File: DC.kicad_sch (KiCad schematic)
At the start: 89 parts, among them J1 348302001, J2 348302001, J3 757570141, J4 PPTC021LFBN-RC, U6 MCP2551-I-P, U7 NUCLEO-F302R8, U8 100DP6T1B1M1QEH

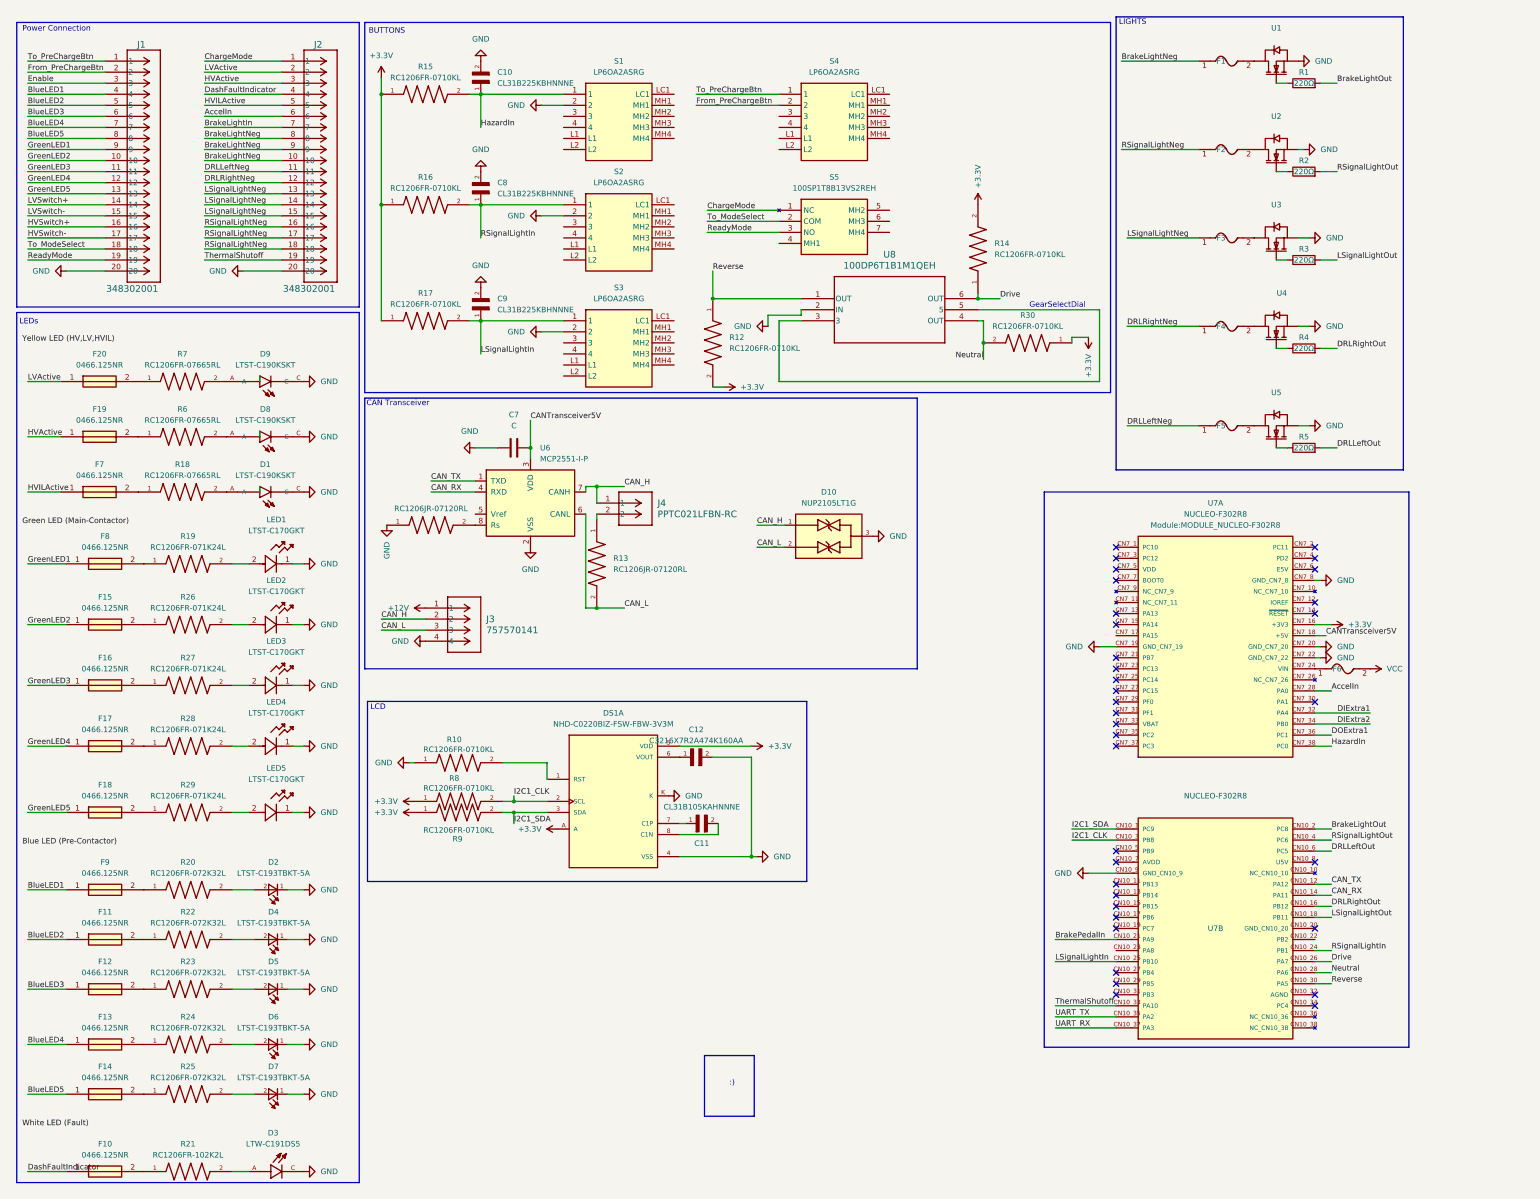
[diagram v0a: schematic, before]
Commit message: VCU revisions, last review still to be done
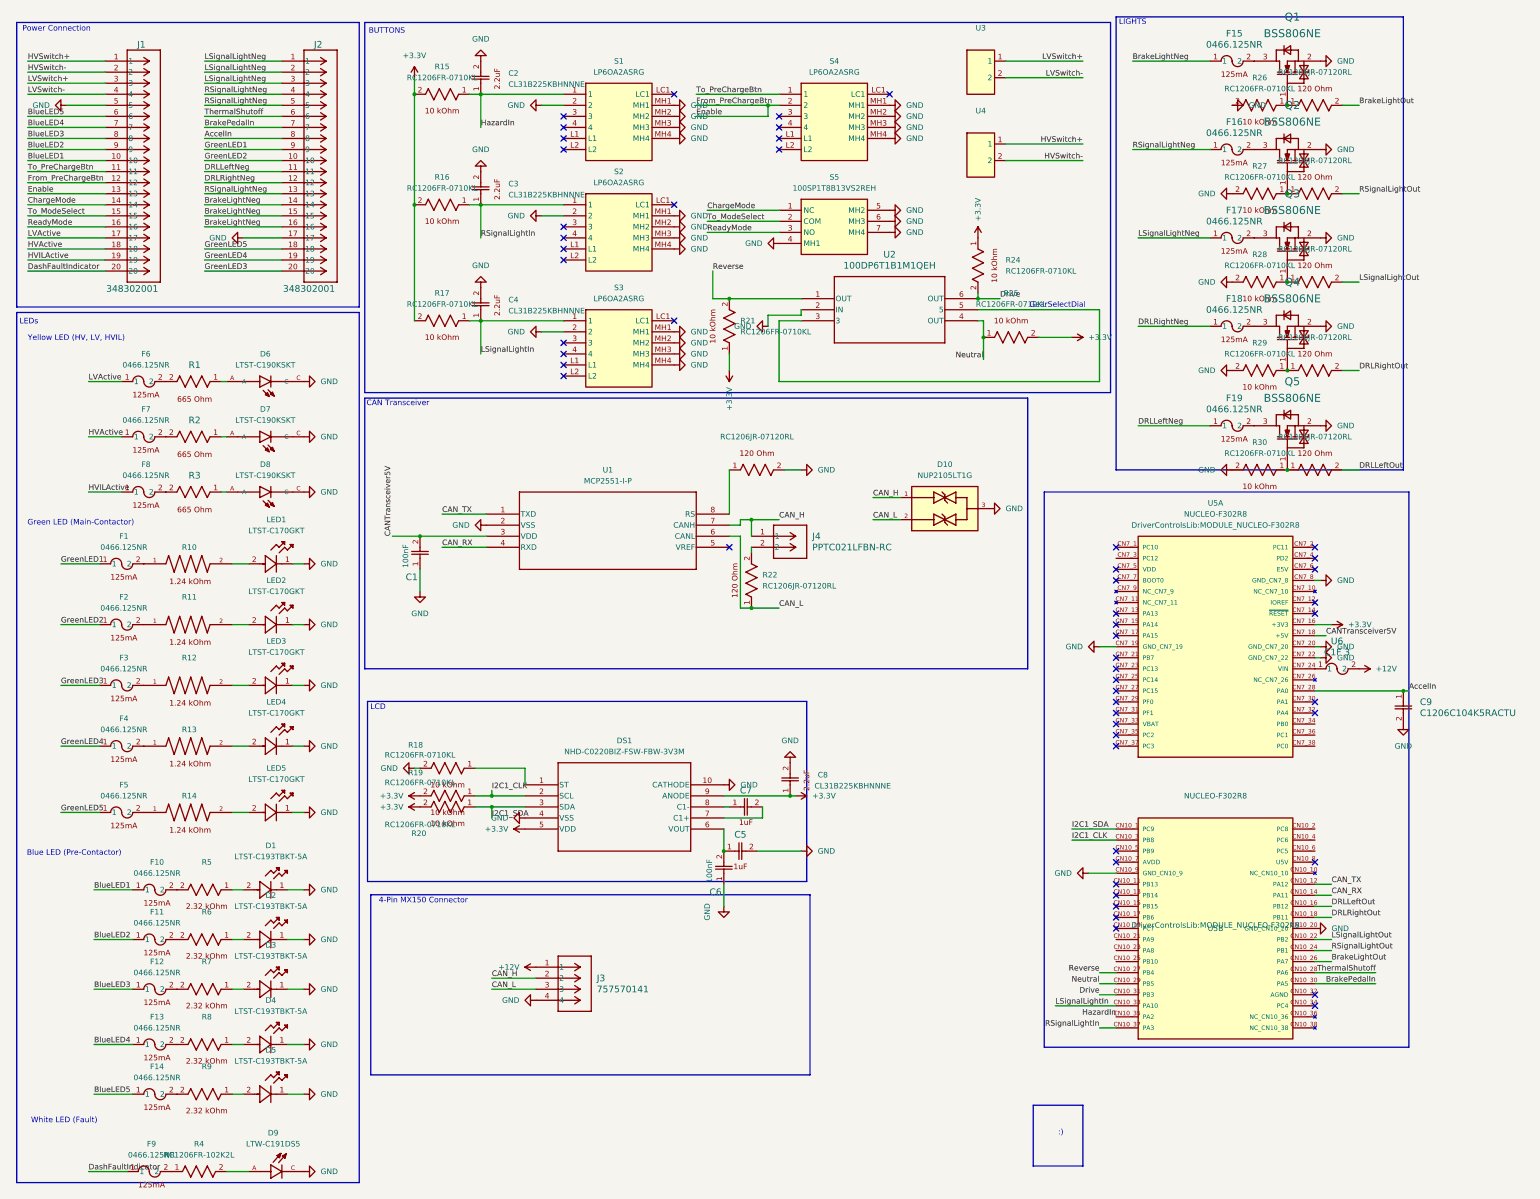
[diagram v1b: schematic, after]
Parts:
- removed C11: CL31B105KAHNNNE, Capacitor_SMD:CAPC3216X180N, symbol CL31B105KAHNNNE:CL31B105KAHNNNE
- removed C12: C3216X7R2A474K160AA, Capacitor_SMD:CAPC3216X180N, symbol C3216X7R2A474K160AA:C3216X7R2A474K160AA
- removed C7: C, DriverControlsLib:CAP-TH_L6.0-W3.5-P7.50-D1.0, symbol DC_Parts:C
- removed F1, F2, F3, F6: ~, DriverControlsLib:FUSE-TH_BD5.4-W22.5-P27.5-D0.8, symbol DC_Parts:0001.2511.TR
- removed F4, F5: ~, Fuse:FUSC3215X66N, symbol DC_Parts:0001.2511.TR
- removed J4: PPTC021LFBN-RC, Connector:CONN2_LFBN-RC_SUL, symbol 2026-02-13_01-22-03:PPTC021LFBN-RC
- removed R1, R2, R3, R4, R5: 220Ω, Resistor_SMD:RESC3216X70N, symbol DC_Parts:R
- removed R18, R6, R7: RC1206FR-07665RL, Resistor_SMD:RESC3116X65N, symbol RC1206FR-07665RL:RC1206FR-07665RL
- removed S1, S2, S3, S4: LP6OA2ASRG, Button_Switch_SMD:LP6OA2ASRG, symbol LP6OA2ASRG:LP6OA2ASRG
- removed S5: 100SP1T8B13VS2REH, Button_Switch_SMD:100SP1T8B13VS2REH, symbol 100SP1T8B13VS2REH:100SP1T8B13VS2REH
- removed U1, U2, U3, U4, U5: ~, Battery:TO254P470X1016X2019-3P, symbol DC_Parts:FQP30N06L
- removed U8: 100DP6T1B1M1QEH, MiscellaneousLibrary:TO_1M1QEH_EWI, symbol Gear-Select-Dial:100DP6T1B1M1QEH
- added C1, C6, C9: C1206C104K5RACTU, DriverControlsLib:CAPC340180_88N_KEM, symbol DriverControlsLib:C1206C104K5RACTU
- added C5, C7: CL31B105KAHNNNE, DriverControlsLib:CAP_CL31_SAM, symbol DriverControlsLib:CL31B105KAHNNNE
- added C8: CL31B225KBHNNNE, DriverControlsLib:CAP_CL31_SAM, symbol DriverControlsLib:CL31B225KBHNNNE
- added F15, F16, F17, F18, F19: 0466.125NR, DriverControlsLib:0466Series_LTF, symbol DriverControlsLib:0466.125NR
- added J4: PPTC021LFBN-RC, DriverControlsLib:CONN2_LFBN-RC_SUL, symbol DriverControlsLib:PPTC021LFBN-RC
- added Q1, Q2, Q3, Q4, Q5: BSS806NE, DriverControlsLib:SOT95P240X110-3N-1-V1, symbol DriverControlsLib:BSS806NE
- added R1, R2, R3: RC1206FR-07665RL, DriverControlsLib:RC1206N_YAG, symbol DriverControlsLib:RC1206FR-07665RL
- added R26, R27, R28, R29, R30: RC1206FR-0710KL, DriverControlsLib:RC1206N_YAG, symbol DriverControlsLib:RC1206FR-0710KL
- added R31, R32, R33, R34, R35: RC1206JR-07120RL, DriverControlsLib:RC1206N_YAG, symbol DriverControlsLib:RC1206JR-07120RL
- added S1, S2, S3, S4: LP6OA2ASRG, DriverControlsLib:LP6OA2ASRG, symbol DriverControlsLib:LP6OA2ASRG
- added S5: 100SP1T8B13VS2REH, DriverControlsLib:100SP1T8B13VS2REH, symbol DriverControlsLib:100SP1T8B13VS2REH
- added U2: 100DP6T1B1M1QEH, DriverControlsLib:TO_1M1QEH_EWI, symbol DriverControlsLib:100DP6T1B1M1QEH
- added U3: ~, DriverControlsLib:LV_Switch, symbol DriverControlsLib:LV_Switch
- added U4: ~, DriverControlsLib:HV_Switch, symbol DriverControlsLib:HV_Switch
- added U6: C1F 3, DriverControlsLib:C1_BEL, symbol DriverControlsLib:C1F_3
- C2: renamed from C10; footprint Capacitor_SMD:CAPC3216X180N -> DriverControlsLib:CAP_CL31_SAM; symbol CL31B225KBHNNNE:CL31B225KBHNNNE -> DriverControlsLib:CL31B225KBHNNNE
- C3: renamed from C8; footprint Capacitor_SMD:CAPC3216X180N -> DriverControlsLib:CAP_CL31_SAM; symbol CL31B225KBHNNNE:CL31B225KBHNNNE -> DriverControlsLib:CL31B225KBHNNNE
- C4: renamed from C9; footprint Capacitor_SMD:CAPC3216X180N -> DriverControlsLib:CAP_CL31_SAM; symbol CL31B225KBHNNNE:CL31B225KBHNNNE -> DriverControlsLib:CL31B225KBHNNNE
- D1: renamed from D2; footprint Fuse:Fuse_0603_1608Metric -> DriverControlsLib:LED_LTST-C_LTO; symbol LTST-C193TBKT-5A:LTST-C193TBKT-5A -> DriverControlsLib:LTST-C193TBKT-5A
- D2: renamed from D4; footprint Fuse:Fuse_0603_1608Metric -> DriverControlsLib:LED_LTST-C_LTO; symbol LTST-C193TBKT-5A:LTST-C193TBKT-5A -> DriverControlsLib:LTST-C193TBKT-5A
- D3: renamed from D5; footprint Fuse:Fuse_0603_1608Metric -> DriverControlsLib:LED_LTST-C_LTO; symbol LTST-C193TBKT-5A:LTST-C193TBKT-5A -> DriverControlsLib:LTST-C193TBKT-5A
- D4: renamed from D6; footprint Fuse:Fuse_0603_1608Metric -> DriverControlsLib:LED_LTST-C_LTO; symbol LTST-C193TBKT-5A:LTST-C193TBKT-5A -> DriverControlsLib:LTST-C193TBKT-5A
- D5: renamed from D7; footprint Fuse:Fuse_0603_1608Metric -> DriverControlsLib:LED_LTST-C_LTO; symbol LTST-C193TBKT-5A:LTST-C193TBKT-5A -> DriverControlsLib:LTST-C193TBKT-5A
- D6: renamed from D9; footprint LED_SMD:LEDM1608X80 -> DriverControlsLib:LEDM1608X80; symbol LTST-C190KSKT:LTST-C190KSKT -> DriverControlsLib:LTST-C190KSKT
- D7: renamed from D8; footprint LED_SMD:LEDM1608X80 -> DriverControlsLib:LEDM1608X80; symbol LTST-C190KSKT:LTST-C190KSKT -> DriverControlsLib:LTST-C190KSKT
- D8: renamed from D1; footprint LED_SMD:LEDM1608X80 -> DriverControlsLib:LEDM1608X80; symbol LTST-C190KSKT:LTST-C190KSKT -> DriverControlsLib:LTST-C190KSKT
- D9: renamed from D3; footprint LED_SMD:LEDC1608X65N -> DriverControlsLib:LEDC1608X65N; symbol LTW-C191DS5:LTW-C191DS5 -> DriverControlsLib:LTW-C191DS5
- DS1: footprint Display:LCD_NHD-C0220BIZ-FSW-FBW-3V3M -> DriverControlsLib:NHD-C0220BIZ-FSW-FBW-3V3M_NDI; symbol NHD-C0220BIZ-FSW-FBW-3V3M:NHD-C0220BIZ-FSW-FBW-3V3M -> DriverControlsLib:NHD-C0220BIZ-FSW-FBW-3V3M
- F1: renamed from F8; footprint Fuse:FUSC3215X66N -> DriverControlsLib:0466Series_LTF; symbol 0466_125NR:0466.125NR -> DriverControlsLib:0466.125NR
- F10: renamed from F9; footprint Fuse:FUSC3215X66N -> DriverControlsLib:0466Series_LTF; symbol 0466_125NR:0466.125NR -> DriverControlsLib:0466.125NR
- F11, F12, F13, F14: footprint Fuse:FUSC3215X66N -> DriverControlsLib:0466Series_LTF; symbol 0466_125NR:0466.125NR -> DriverControlsLib:0466.125NR
- F2: renamed from F15; footprint Fuse:FUSC3215X66N -> DriverControlsLib:0466Series_LTF; symbol 0466_125NR:0466.125NR -> DriverControlsLib:0466.125NR
- F3: renamed from F16; footprint Fuse:FUSC3215X66N -> DriverControlsLib:0466Series_LTF; symbol 0466_125NR:0466.125NR -> DriverControlsLib:0466.125NR
- F4: renamed from F17; footprint Fuse:FUSC3215X66N -> DriverControlsLib:0466Series_LTF; symbol 0466_125NR:0466.125NR -> DriverControlsLib:0466.125NR
- F5: renamed from F18; footprint Fuse:FUSC3215X66N -> DriverControlsLib:0466Series_LTF; symbol 0466_125NR:0466.125NR -> DriverControlsLib:0466.125NR
- F6: renamed from F20; footprint Fuse:FUSC3215X66N -> DriverControlsLib:0466Series_LTF; symbol 0466_125NR:0466.125NR -> DriverControlsLib:0466.125NR
- F7: renamed from F19; footprint Fuse:FUSC3215X66N -> DriverControlsLib:0466Series_LTF; symbol 0466_125NR:0466.125NR -> DriverControlsLib:0466.125NR
- F8: renamed from F7; footprint Fuse:FUSC3215X66N -> DriverControlsLib:0466Series_LTF; symbol 0466_125NR:0466.125NR -> DriverControlsLib:0466.125NR
- F9: renamed from F10; footprint Fuse:FUSC3215X66N -> DriverControlsLib:0466Series_LTF; symbol 0466_125NR:0466.125NR -> DriverControlsLib:0466.125NR
- J1, J2: footprint Connector_Molex:CONN_SD-34829-001_20_ST_MOL -> DriverControlsLib:CONN_SD-34829-001_20_ST_MOL; symbol MX150_sym:348302001 -> DriverControlsLib:348302001
- J3: footprint Connector_Molex:CONN_SD-75757-010_1X4_F11p20_MOL -> DriverControlsLib:CONN_SD-75757-010_1X4_F11p20_MOL; symbol 2026-02-11_03-05-32:757570141 -> DriverControlsLib:757570141
- LED1, LED2, LED3, LED4, LED5: footprint LED_SMD:LED_LTST-C170GKT_LTO -> DriverControlsLib:LED_LTST-C170GKT_LTO; symbol 2026-02-10_18-36-51:LTST-C170GKT -> DriverControlsLib:LTST-C170GKT
- R10: renamed from R19; footprint Resistor_SMD:RESC3116X65N -> DriverControlsLib:RESC3116X65N; symbol RC1206FR-071K24L:RC1206FR-071K24L -> DriverControlsLib:RC1206FR-071K24L
- R11: renamed from R26; footprint Resistor_SMD:RESC3116X65N -> DriverControlsLib:RESC3116X65N; symbol RC1206FR-071K24L:RC1206FR-071K24L -> DriverControlsLib:RC1206FR-071K24L
- R12: renamed from R27; footprint Resistor_SMD:RESC3116X65N -> DriverControlsLib:RESC3116X65N; symbol RC1206FR-071K24L:RC1206FR-071K24L -> DriverControlsLib:RC1206FR-071K24L
- R13: renamed from R28; footprint Resistor_SMD:RESC3116X65N -> DriverControlsLib:RESC3116X65N; symbol RC1206FR-071K24L:RC1206FR-071K24L -> DriverControlsLib:RC1206FR-071K24L
- R14: renamed from R29; footprint Resistor_SMD:RESC3116X65N -> DriverControlsLib:RESC3116X65N; symbol RC1206FR-071K24L:RC1206FR-071K24L -> DriverControlsLib:RC1206FR-071K24L
- R15, R16, R17: footprint Resistor_SMD:RESC3116X65N -> DriverControlsLib:RC1206N_YAG; symbol RC1206FR-0710KL:RC1206FR-0710KL -> DriverControlsLib:RC1206FR-0710KL
- R18: renamed from R10; footprint Resistor_SMD:RESC3116X65N -> DriverControlsLib:RC1206N_YAG; symbol RC1206FR-0710KL:RC1206FR-0710KL -> DriverControlsLib:RC1206FR-0710KL
- R19: renamed from R8; footprint Resistor_SMD:RESC3116X65N -> DriverControlsLib:RC1206N_YAG; symbol RC1206FR-0710KL:RC1206FR-0710KL -> DriverControlsLib:RC1206FR-0710KL
- R20: renamed from R9; footprint Resistor_SMD:RESC3116X65N -> DriverControlsLib:RC1206N_YAG; symbol RC1206FR-0710KL:RC1206FR-0710KL -> DriverControlsLib:RC1206FR-0710KL
- R21: renamed from R12; footprint MiscellaneousLibrary:RESC3116X65N -> DriverControlsLib:RC1206N_YAG; symbol RC1206FR-0710KL:RC1206FR-0710KL -> DriverControlsLib:RC1206FR-0710KL
- R22: renamed from R13; footprint Resistor_SMD:RESC3116X65N -> DriverControlsLib:RC1206N_YAG; symbol RC1206JR-07120RL:RC1206JR-07120RL -> DriverControlsLib:RC1206JR-07120RL
- R23: renamed from R11; footprint Resistor_SMD:RESC3116X65N -> DriverControlsLib:RC1206N_YAG; symbol RC1206JR-07120RL:RC1206JR-07120RL -> DriverControlsLib:RC1206JR-07120RL
- R24: renamed from R14; footprint MiscellaneousLibrary:RESC3116X65N -> DriverControlsLib:RC1206N_YAG; symbol RC1206FR-0710KL:RC1206FR-0710KL -> DriverControlsLib:RC1206FR-0710KL
- R25: renamed from R30; footprint MiscellaneousLibrary:RESC3116X65N -> DriverControlsLib:RC1206N_YAG; symbol RC1206FR-0710KL:RC1206FR-0710KL -> DriverControlsLib:RC1206FR-0710KL
- R4: renamed from R21; footprint Resistor_SMD:RESC3116X65N -> DriverControlsLib:RES_RC1206_YAG; symbol RC1206FR-102K2L:RC1206FR-102K2L -> DriverControlsLib:RC1206FR-102K2L
- R5: renamed from R20; footprint Resistor_SMD:RESC3116X65N -> DriverControlsLib:RC1206N_YAG; symbol RC1206FR-072K32L:RC1206FR-072K32L -> DriverControlsLib:RC1206FR-072K32L
- R6: renamed from R22; footprint Resistor_SMD:RESC3116X65N -> DriverControlsLib:RC1206N_YAG; symbol RC1206FR-072K32L:RC1206FR-072K32L -> DriverControlsLib:RC1206FR-072K32L
- R7: renamed from R23; footprint Resistor_SMD:RESC3116X65N -> DriverControlsLib:RC1206N_YAG; symbol RC1206FR-072K32L:RC1206FR-072K32L -> DriverControlsLib:RC1206FR-072K32L
- R8: renamed from R24; footprint Resistor_SMD:RESC3116X65N -> DriverControlsLib:RC1206N_YAG; symbol RC1206FR-072K32L:RC1206FR-072K32L -> DriverControlsLib:RC1206FR-072K32L
- R9: renamed from R25; footprint Resistor_SMD:RESC3116X65N -> DriverControlsLib:RC1206N_YAG; symbol RC1206FR-072K32L:RC1206FR-072K32L -> DriverControlsLib:RC1206FR-072K32L
- U1: renamed from U6; footprint Package_DIP:DIP-8_W7.62mm -> DriverControlsLib:PDIP8_300MC_MCH; symbol DC_Parts:MCP2551-I-P -> DriverControlsLib:MCP2551-I_P
- U5: renamed from U7; footprint Module:MODULE_NUCLEO-F302R8 -> DriverControlsLib:MODULE_NUCLEO-F302R8; symbol DC_Parts:NUCLEO-F302R8 -> DriverControlsLib:NUCLEO-F302R8
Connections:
- net BrakeLightIn is gone; now on net BrakePedalIn: J2.7
- net From_PreChargeBtn is gone; now on net HVSwitch-: J1.2
- net UART_RX is gone; now on net RSignalLightIn: U5.CN10_37 (PA3)
- net UART_TX is gone; now on net HazardIn: U5.CN10_35 (PA2)
- net +12V: now also U6.2
- net +3.3V: now also DS1.9 (ANODE), R15.2, R16.2, R17.2, R19.2, R20.2, R21.1, R24.1, R25.2, C8.1; no longer DS1.A, R15.1, R16.1, R17.1, R19.1, R20.1, R21.2, R24.2, R25.1
- net AccelIn: now also J2.8, C9.1; no longer J2.6
- net BlueLED1: now also J1.10; no longer J1.4
- net BlueLED2: now also J1.9; no longer J1.5
- net BlueLED3: now also J1.8; no longer J1.6
- net BlueLED5: now also J1.6; no longer J1.8
- net BrakeLightNeg: now also J2.14, J2.15, J2.16, F15.1; no longer J2.10, J2.8, J2.9
- net BrakeLightOut: now also U5.CN10_26 (PA7), R31.2; no longer U5.CN10_2 (PC8)
- net BrakePedalIn: now also U5.CN10_30 (PA5); no longer U5.CN10_21 (PA9)
- net CANTransceiver5V: now also C1.2
- net CAN_H: now also J4.1
- net CAN_L: now also R22.1; no longer R22.2
- net ChargeMode: now also J1.14, S5.1 (NC); no longer J2.1
- net DRLLeftNeg: now also F19.1
- net DRLLeftOut: now also U5.CN10_16 (PB12), R35.2; no longer U5.CN10_6 (PC5)
- net DRLRightNeg: now also F18.1
- net DRLRightOut: now also U5.CN10_18 (PB11), R34.2; no longer U5.CN10_16 (PB12)
- net DashFaultIndicator: now also J1.20; no longer J2.4
- net Drive: now also R24.2, U5.CN10_31 (PB3), U2.6 (OUT); no longer R24.1, U5.CN10_26 (PA7)
- net Enable: now also J1.12, J1.13, S4.2; no longer J1.3
- net GND: now also DS1.10 (CATHODE), J1.5, J2.17, R18.2, R23.2, U5.CN10_20 (GND_CN10_20), C1.1, C5.2, C6.1, C8.2, C9.2, Q1.2 (SOURCE), Q2.2 (SOURCE), Q3.2 (SOURCE), Q4.2 (SOURCE), Q5.2 (SOURCE), R26.2, R27.2, R28.2, R29.2, R30.2, S1.2, S1.MH1, S1.MH2, S1.MH3, S1.MH4, S2.2, S2.MH1, S2.MH2, S2.MH3, S2.MH4, S3.2, S3.MH1, S3.MH2, S3.MH3, S3.MH4, S4.MH1, S4.MH2, S4.MH3, S4.MH4, S5.4 (MH1), S5.5 (MH2), S5.6 (MH3), S5.7 (MH4), U2.2 (IN); no longer DS1.K, J1.20, J2.20, R18.1, R23.1
- net GreenLED1: now also J2.9; no longer J1.9
- net GreenLED2: now also J2.10; no longer J1.10
- net GreenLED3: now also J2.20; no longer J1.11
- net GreenLED4: now also J2.19; no longer J1.12
- net GreenLED5: now also J2.18; no longer J1.13
- net HVActive: now also J1.18; no longer J2.3
- net HVILActive: now also J1.19; no longer J2.5
- net HVSwitch+: now also J1.1, U4.1; no longer J1.16
- net HVSwitch-: now also U4.2; no longer J1.17
- net HazardIn: now also R15.1, S1.1; no longer R15.2, U5.CN7_38 (PC0)
- net I2C1_CLK: now also R19.1; no longer R19.2
- net I2C1_SDA: now also R20.1; no longer R20.2
- net LSignalLightIn: now also R17.1, U5.CN10_33 (PA10), S3.1; no longer R17.2, U5.CN10_25 (PB10)
- net LSignalLightNeg: now also J2.1, J2.2, J2.3, F17.1; no longer J2.13, J2.14, J2.15
- net LSignalLightOut: now also U5.CN10_22 (PB2), R33.2; no longer U5.CN10_18 (PB11)
- net LVActive: now also J1.17; no longer J2.2
- net LVSwitch+: now also J1.3, U3.1; no longer J1.14
- net LVSwitch-: now also J1.4, U3.2; no longer J1.15
- net Neutral: now also R25.1, U5.CN10_29 (PB5), U2.4 (OUT); no longer R25.2, U5.CN10_28 (PA6)
- net RSignalLightIn: now also R16.1, S2.1; no longer R16.2, U5.CN10_24 (PB1)
- net RSignalLightNeg: now also J2.13, J2.4, J2.5, F16.1; no longer J2.16, J2.17, J2.18
- net RSignalLightOut: now also U5.CN10_24 (PB1), R32.2; no longer U5.CN10_4 (PC6)
- net ReadyMode: now also J1.16, S5.3 (NO); no longer J1.19
- net Reverse: now also R21.2, U5.CN10_27 (PB4), U2.1 (OUT); no longer R21.1, U5.CN10_30 (PA5)
- net ThermalShutoff: now also J2.6, U5.CN10_28 (PA6); no longer J2.19, U5.CN10_33 (PA10)
- net To_ModeSelect: now also J1.15, S5.2 (COM); no longer J1.18
- net To_PreChargeBtn: now also J1.11, S4.1; no longer J1.1
- net at D7.A: now also R2.1
- net at R6.1: now also D2.2; no longer F11.2
- net at R6.2: now also F11.2; no longer D2.2
- net at R9.1: now also D5.2; no longer F14.2
- net at R9.2: now also F14.2; no longer D5.2
- net at F12.2: now also R7.2; no longer R7.1
- net at D8.A: now also R3.1
- net at DS1.1 (ST): now also R18.1; no longer R18.2
- net at F7.2: now also R2.2
- net at F8.2: now also R3.2
- net at R8.1: now also D4.2; no longer F13.2
- net at R8.2: now also F13.2; no longer D4.2
- net at DS1.6 (VOUT): now also C5.1, C6.2
- net at DS1.7 (C1+): now also C7.2
- net at DS1.8 (C1-): now also C7.1
- net at U1.8 (RS): now also R23.1; no longer R23.2
- net at D6.A: now also R1.1
- net at D3.2: now also R7.1; no longer R7.2
- net at U5.CN7_24 (VIN): now also U6.1
- net at R5.1: now also D1.2; no longer F10.2
- net at R5.2: now also F10.2; no longer D1.2
- net at F6.2: now also R1.2
- net DIExtra1: no longer names the net of U5.CN7_32 (PA4)
- net DIExtra2: no longer names the net of U5.CN7_34 (PB0)
- net DOExtra1: no longer names the net of U5.CN7_36 (PC1)
- new net: F19.2, Q5.3 (DRAIN)
- new net: Q5.1 (GATE), R30.1, R35.1
- new net: J4.2, R22.2
- new net: F17.2, Q3.3 (DRAIN)
- new net: Q2.1 (GATE), R27.1, R32.1
- new net: Q3.1 (GATE), R28.1, R33.1
- new net: F15.2, Q1.3 (DRAIN)
- new net: U2.3, U2.5
- new net: F18.2, Q4.3 (DRAIN)
- new net: Q1.1 (GATE), R26.1, R31.1
- new net: F16.2, Q2.3 (DRAIN)
- new net: Q4.1 (GATE), R29.1, R34.1
- no-connect marks 35 -> 53
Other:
- note added: "4-Pin MX150 Connector"
- note added: "Blue LED (Pre-Contactor)"
- note added: "Green LED (Main-Contactor)"
- note added: "White LED (Fault)"
- note added: "Yellow LED (HV, LV, HVIL)"
- moved on the sheet: D10, J3
